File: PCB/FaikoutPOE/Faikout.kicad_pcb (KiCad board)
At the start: 2 copper layers, 42 x 69 mm, 85 parts, among them J1 RJ45_LED, J3 S21, J5 Reset, J7 TC2030-USB-NL-DS, M1 Ag9912-LP, P1 Square, Q1 BSS138PS, Q2 BSS138PS, U1 KSZ8851SNL, U2 ESP32-S3-MINI-1, U3 TCMT1100, U4 TPS62933, U5 TCMT1100, Y1 Crystal_GND24

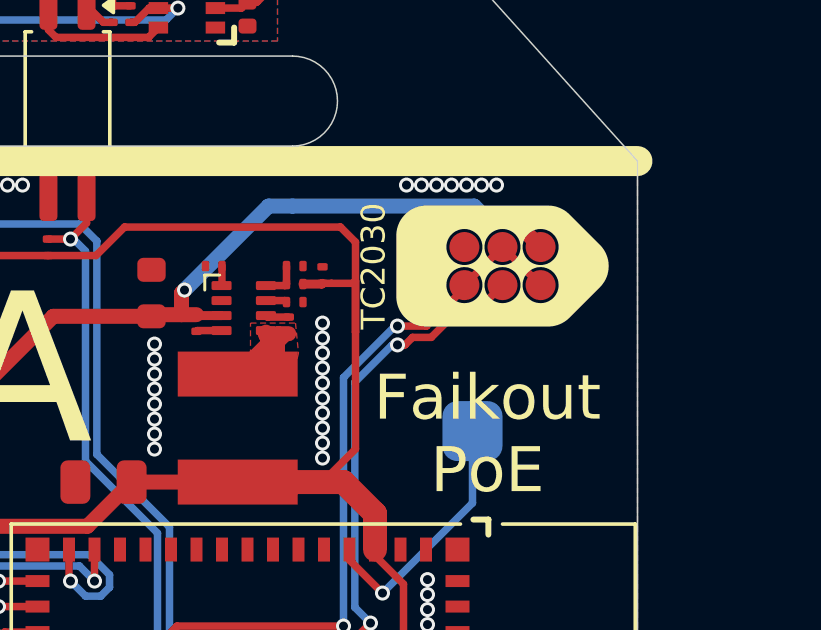
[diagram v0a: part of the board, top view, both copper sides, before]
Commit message: Fix BOM
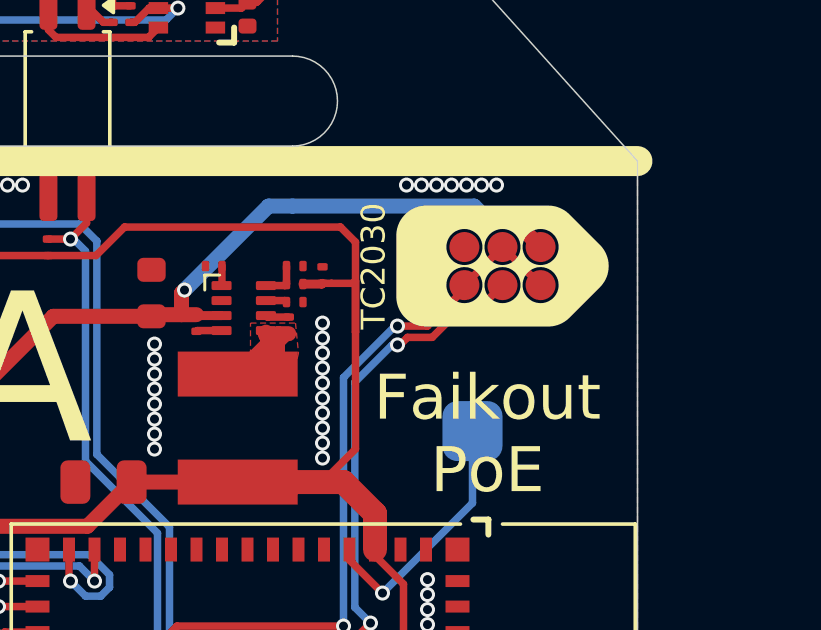
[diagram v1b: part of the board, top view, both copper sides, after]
